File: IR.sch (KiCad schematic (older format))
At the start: 9 parts

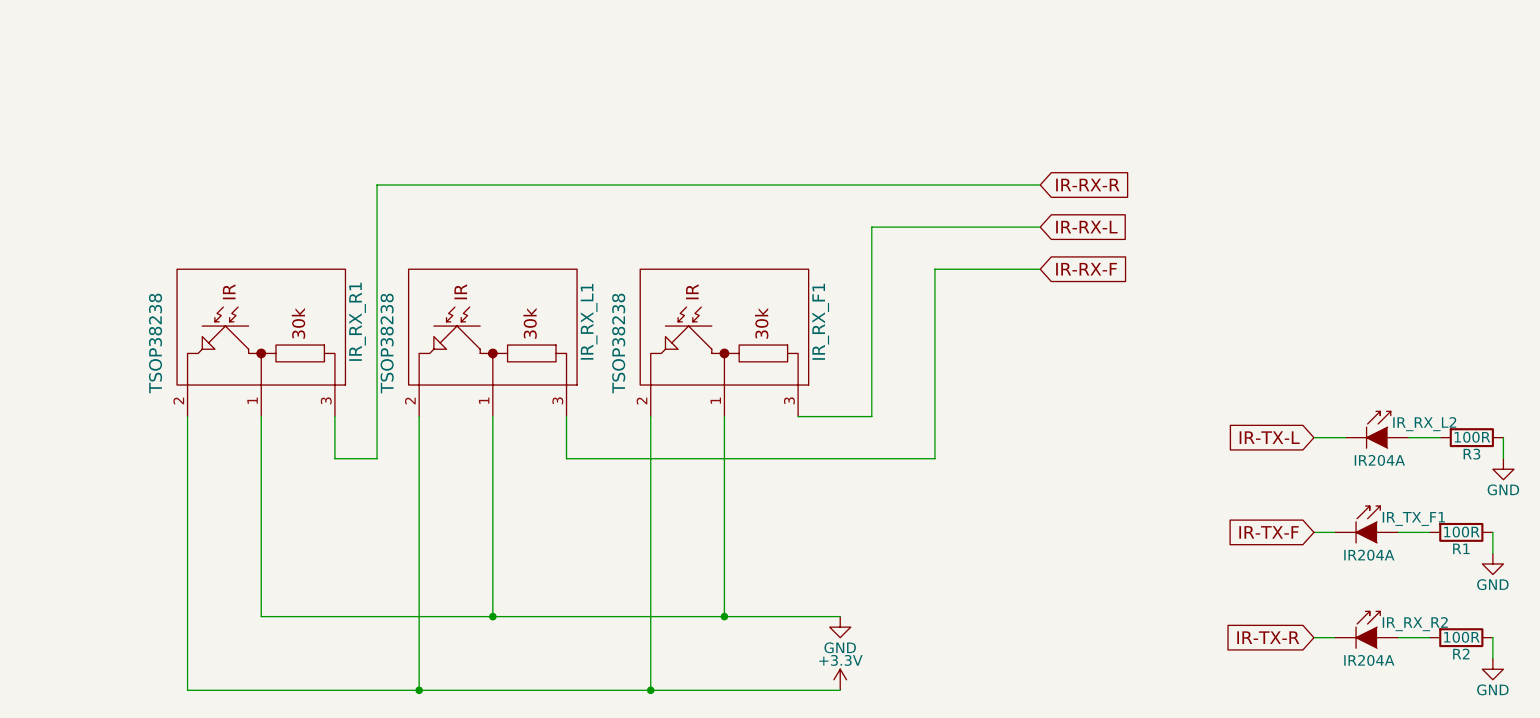
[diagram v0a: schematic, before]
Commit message: Fixed up some mess + IR + USB new footprint + buttons
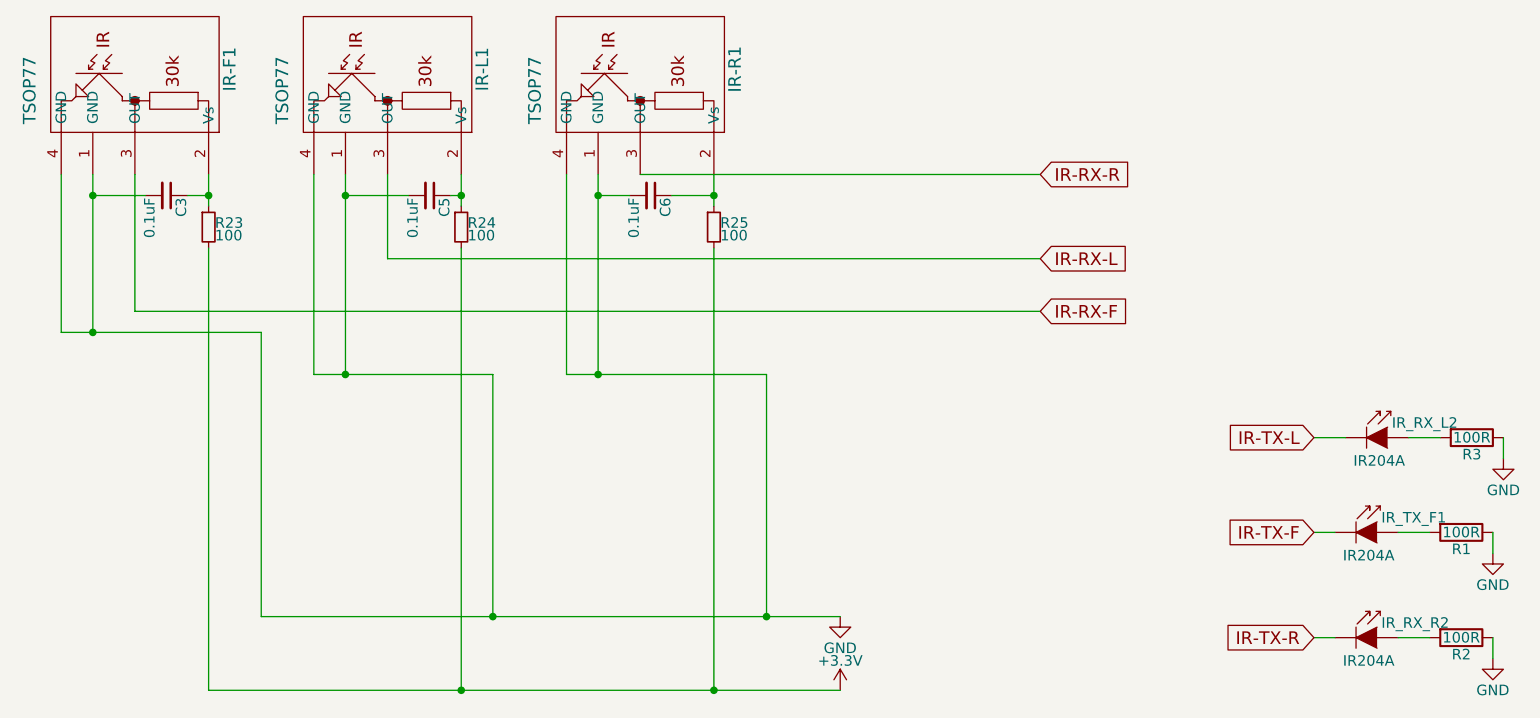
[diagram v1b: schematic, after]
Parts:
- removed IR_RX_F1, IR_RX_L1, IR_RX_R1: TSOP38238, custom-footprints:IR_Receiver, symbol TSOP38238
- added C3, C5, C6: 0.1uF, Capacitors_SMD:C_0603, symbol C_Small
- added IR-F1, IR-L1, IR-R1: TSOP77, tsop77:SOIC-4, symbol TSOP77
- added R23, R24, R25: 100, Resistors_SMD:R_0603, symbol R_Small
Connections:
- net +3V3: now also R23.2, R24.2, R25.2
- net GND: now also C3.2, C5.2, C6.2, IR-F1.1 (GND), IR-F1.4 (GND), IR-L1.1 (GND), IR-L1.4 (GND), IR-R1.1 (GND), IR-R1.4 (GND)
- net IR-RX-F: now also IR-F1.3 (OUT)
- net IR-RX-L: now also IR-L1.3 (OUT)
- net IR-RX-R: now also IR-R1.3 (OUT)
- new net: C3.1, IR-F1.2 (Vs), R23.1
- new net: C5.1, IR-L1.2 (Vs), R24.1
- new net: C6.1, IR-R1.2 (Vs), R25.1
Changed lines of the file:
@@
 $EndDescr
 $Comp
-L TSOP38238 IR_RX_F1
-U 1 1 5B14511A
-P 4350 3400
-F 0 "IR_RX_F1" H 4300 3850 60  0000 C CNN
-F 1 "TSOP38238" H 4400 2900 60  0000 C CNN
-F 2 "custom-footprints:IR_Receiver" H 4350 3400 60  0001 C CNN
-F 3 "" H 4350 3400 60  0001 C CNN
-	1    4350 3400
-	0    1    1    0
-$EndComp
-$Comp
-L TSOP38238 IR_RX_L1
-U 1 1 5B145121
-P 3250 3400
-F 0 "IR_RX_L1" H 3200 3850 60  0000 C CNN
-F 1 "TSOP38238" H 3300 2900 60  0000 C CNN
-F 2 "custom-footprints:IR_Receiver" H 3250 3400 60  0001 C CNN
-F 3 "" H 3250 3400 60  0001 C CNN
-	1    3250 3400
-	0    1    1    0
-$EndComp
-$Comp
-L TSOP38238 IR_RX_R1
-U 1 1 5B145128
-P 2150 3400
-F 0 "IR_RX_R1" H 2100 3850 60  0000 C CNN
-F 1 "TSOP38238" H 2200 2900 60  0000 C CNN
-F 2 "custom-footprints:IR_Receiver" H 2150 3400 60  0001 C CNN
-F 3 "" H 2150 3400 60  0001 C CNN
-	1    2150 3400
-	0    1    1    0
-$EndComp
-$Comp
-L GND #PWR1228
+L GND #PWR1229
 U 1 1 5B14512F
 P 4900 4750
-F 0 "#PWR1228" H 4900 4500 50  0001 C CNN
+F 0 "#PWR1229" H 4900 4500 50  0001 C CNN
 F 1 "GND" H 4900 4600 50  0000 C CNN
 F 2 "" H 4900 4750 50  0001 C CNN
@@
 $EndComp
 $Comp
-L GND #PWR1230
+L GND #PWR1231
 U 1 1 5B14515F
 P 8000 4450
-F 0 "#PWR1230" H 8000 4200 50  0001 C CNN
+F 0 "#PWR1231" H 8000 4200 50  0001 C CNN
 F 1 "GND" H 8000 4300 50  0000 C CNN
 F 2 "" H 8000 4450 50  0001 C CNN
@@
 $EndComp
 $Comp
-L GND #PWR1232
+L GND #PWR1233
 U 1 1 5B145165
 P 8050 4000
-F 0 "#PWR1232" H 8050 3750 50  0001 C CNN
+F 0 "#PWR1233" H 8050 3750 50  0001 C CNN
 F 1 "GND" H 8050 3850 50  0000 C CNN
 F 2 "" H 8050 4000 50  0001 C CNN
@@
 $EndComp
 $Comp
-L GND #PWR1231
+L GND #PWR1232
 U 1 1 5B14516B
 P 8000 4950
-F 0 "#PWR1231" H 8000 4700 50  0001 C CNN
+F 0 "#PWR1232" H 8000 4700 50  0001 C CNN
 F 1 "GND" H 8000 4800 50  0000 C CNN
 F 2 "" H 8000 4950 50  0001 C CNN
@@
 $EndComp
 Wire Wire Line
-	4000 3800 4000 5100
-Wire Wire Line
-	1800 5100 4900 5100
-Wire Wire Line
-	2900 5100 2900 3800
-Connection ~ 4000 5100
-Wire Wire Line
-	1800 5100 1800 3800
-Connection ~ 2900 5100
-Wire Wire Line
-	4350 4750 4350 3800
-Wire Wire Line
 	2150 4750 4900 4750
 Wire Wire Line
-	3250 4750 3250 3800
-Connection ~ 4350 4750
-Wire Wire Line
-	2150 4750 2150 3800
-Connection ~ 3250 4750
-Wire Wire Line
 	8000 4350 8000 4450
 Wire Wire Line
@@
 	8000 4850 8000 4950
 Wire Wire Line
-	5050 3800 4700 3800
-Wire Wire Line
-	5050 2900 5050 3800
-Wire Wire Line
-	3600 3800 3600 4000
-Wire Wire Line
-	2500 3800 2500 4000
-Wire Wire Line
 	7550 4350 7700 4350
 Wire Wire Line
@@
 Wire Wire Line
 	7550 4850 7700 4850
-Wire Wire Line
-	5850 2900 5050 2900
-Wire Wire Line
-	3600 4000 5350 4000
-Wire Wire Line
-	5350 4000 5350 3100
-Wire Wire Line
-	5350 3100 5850 3100
-Wire Wire Line
-	2500 4000 2700 4000
-Wire Wire Line
-	2700 4000 2700 2700
-Wire Wire Line
-	2700 2700 5850 2700
-$Comp
-L +3.3V #PWR1229
+$Comp
+L +3.3V #PWR1230
 U 1 1 5B14519E
 P 4900 5100
-F 0 "#PWR1229" H 4900 4950 50  0001 C CNN
+F 0 "#PWR1230" H 4900 4950 50  0001 C CNN
 F 1 "+3.3V" H 4900 5240 50  0000 C CNN
 F 2 "" H 4900 5100 50  0001 C CNN
@@
 	1    0    0    -1
 $EndComp
-Text GLabel 5850 2700 2    60   Input ~ 0
+Text GLabel 5850 2650 2    60   Input ~ 0
 IR-RX-R
-Text GLabel 5850 2900 2    60   Input ~ 0
+Text GLabel 5850 3050 2    60   Input ~ 0
 IR-RX-L
-Text GLabel 5850 3100 2    60   Input ~ 0
+Text GLabel 5850 3300 2    60   Input ~ 0
 IR-RX-F
 Text GLabel 7150 3900 0    60   Input ~ 0
@@
 Wire Wire Line
 	7150 4850 7250 4850
+$Comp
+L R_Small R23
+U 1 1 5B16CE8C
+P 1900 2900
+F 0 "R23" H 1930 2920 50  0000 L CNN
+F 1 "100" H 1930 2860 50  0000 L CNN
+F 2 "Resistors_SMD:R_0603" H 1900 2900 50  0001 C CNN
+F 3 "" H 1900 2900 50  0001 C CNN
+	1    1900 2900
+	1    0    0    -1
+$EndComp
+$Comp
+L R_Small R24
+U 1 1 5B16D0F7
+P 3100 2900
+F 0 "R24" H 3130 2920 50  0000 L CNN
+F 1 "100" H 3130 2860 50  0000 L CNN
+F 2 "Resistors_SMD:R_0603" H 3100 2900 50  0001 C CNN
+F 3 "" H 3100 2900 50  0001 C CNN
+	1    3100 2900
+	1    0    0    -1
+$EndComp
+$Comp
+L R_Small R25
+U 1 1 5B16D14B
+P 4300 2900
+F 0 "R25" H 4330 2920 50  0000 L CNN
+F 1 "100" H 4330 2860 50  0000 L CNN
+F 2 "Resistors_SMD:R_0603" H 4300 2900 50  0001 C CNN
+F 3 "" H 4300 2900 50  0001 C CNN
+	1    4300 2900
+	1    0    0    -1
+$EndComp
+$Comp
+L TSOP77 IR-F1
+U 1 1 5B16D249
+P 1550 2200
+F 0 "IR-F1" H 1500 2650 60  0000 C CNN
+F 1 "TSOP77" H 1600 1700 60  0000 C CNN
+F 2 "tsop77:SOIC-4" H 1550 2200 60  0001 C CNN
+F 3 "" H 1550 2200 60  0001 C CNN
+	1    1550 2200
+	0    1    1    0
+$EndComp
+$Comp
+L TSOP77 IR-L1
+U 1 1 5B16D482
+P 2750 2200
+F 0 "IR-L1" H 2700 2650 60  0000 C CNN
+F 1 "TSOP77" H 2800 1700 60  0000 C CNN
+F 2 "tsop77:SOIC-4" H 2750 2200 60  0001 C CNN
+F 3 "" H 2750 2200 60  0001 C CNN
+	1    2750 2200
+	0    1    1    0
+$EndComp
+$Comp
+L TSOP77 IR-R1
+U 1 1 5B16D4DD
+P 3950 2200
+F 0 "IR-R1" H 3900 2650 60  0000 C CNN
+F 1 "TSOP77" H 4000 1700 60  0000 C CNN
+F 2 "tsop77:SOIC-4" H 3950 2200 60  0001 C CNN
+F 3 "" H 3950 2200 60  0001 C CNN
+	1    3950 2200
+	0    1    1    0
+$EndComp
+Wire Wire Line
+	1200 2650 1200 3400
+Wire Wire Line
+	1200 3400 2150 3400
+Wire Wire Line
+	1350 2650 1350 3400
+Connection ~ 1350 3400
+Wire Wire Line
+	2400 2650 2400 3600
+Wire Wire Line
+	2400 3600 3250 3600
+Wire Wire Line
+	2550 2650 2550 3600
+Connection ~ 2550 3600
+Wire Wire Line
+	3600 2650 3600 3600
+Wire Wire Line
+	3750 2650 3750 3600
+Wire Wire Line
+	1900 5100 4900 5100
+Connection ~ 4300 5100
+Connection ~ 3100 5100
+Wire Wire Line
+	3600 3600 4550 3600
+Connection ~ 4550 4750
+Connection ~ 3750 3600
+Wire Wire Line
+	2150 3400 2150 4750
+Wire Wire Line
+	3250 3600 3250 4750
+Connection ~ 3250 4750
+Wire Wire Line
+	1900 2650 1900 2800
+Wire Wire Line
+	1900 3000 1900 5100
+Wire Wire Line
+	3100 2650 3100 2800
+Wire Wire Line
+	3100 3000 3100 5100
+Wire Wire Line
+	4300 2650 4300 2800
+Wire Wire Line
+	4300 3000 4300 5100
+Wire Wire Line
+	4550 3600 4550 4750
+Wire Wire Line
+	3950 2650 5850 2650
+Wire Wire Line
+	1550 2650 1550 3300
+Wire Wire Line
+	1550 3300 5850 3300
+Wire Wire Line
+	2750 2650 2750 3050
+Wire Wire Line
+	2750 3050 5850 3050
+$Comp
+L C_Small C6
+U 1 1 5B16E22B
+P 4000 2750
+F 0 "C6" H 4010 2820 50  0000 L CNN
+F 1 "0.1uF" H 4010 2670 50  0000 L CNN
+F 2 "Capacitors_SMD:C_0603" H 4000 2750 50  0001 C CNN
+F 3 "" H 4000 2750 50  0001 C CNN
+	1    4000 2750
+	0    1    1    0
+$EndComp
+$Comp
+L C_Small C5
+U 1 1 5B16E3ED
+P 2950 2750
+F 0 "C5" H 2960 2820 50  0000 L CNN
+F 1 "0.1uF" H 2960 2670 50  0000 L CNN
+F 2 "Capacitors_SMD:C_0603" H 2950 2750 50  0001 C CNN
+F 3 "" H 2950 2750 50  0001 C CNN
+	1    2950 2750
+	0    1    1    0
+$EndComp
+$Comp
+L C_Small C3
+U 1 1 5B16E44D
+P 1700 2750
+F 0 "C3" H 1710 2820 50  0000 L CNN
+F 1 "0.1uF" H 1710 2670 50  0000 L CNN
+F 2 "Capacitors_SMD:C_0603" H 1700 2750 50  0001 C CNN
+F 3 "" H 1700 2750 50  0001 C CNN
+	1    1700 2750
+	0    1    1    0
+$EndComp
+Wire Wire Line
+	4100 2750 4300 2750
+Connection ~ 4300 2750
+Wire Wire Line
+	3900 2750 3750 2750
+Connection ~ 3750 2750
+Wire Wire Line
+	3050 2750 3100 2750
+Connection ~ 3100 2750
+Wire Wire Line
+	2850 2750 2550 2750
+Connection ~ 2550 2750
+Wire Wire Line
+	1800 2750 1900 2750
+Connection ~ 1900 2750
+Wire Wire Line
+	1600 2750 1350 2750
+Connection ~ 1350 2750
 $EndSCHEMATC
